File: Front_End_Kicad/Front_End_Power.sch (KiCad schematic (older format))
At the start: 26 parts, among them J201 Conn_01x01_Male, J202 Barrel_Jack, J203 Conn_01x01_Male, SW201 SW_DIP_x01, U201 MAX871, U202 AZ1117IH-5.0TRG1

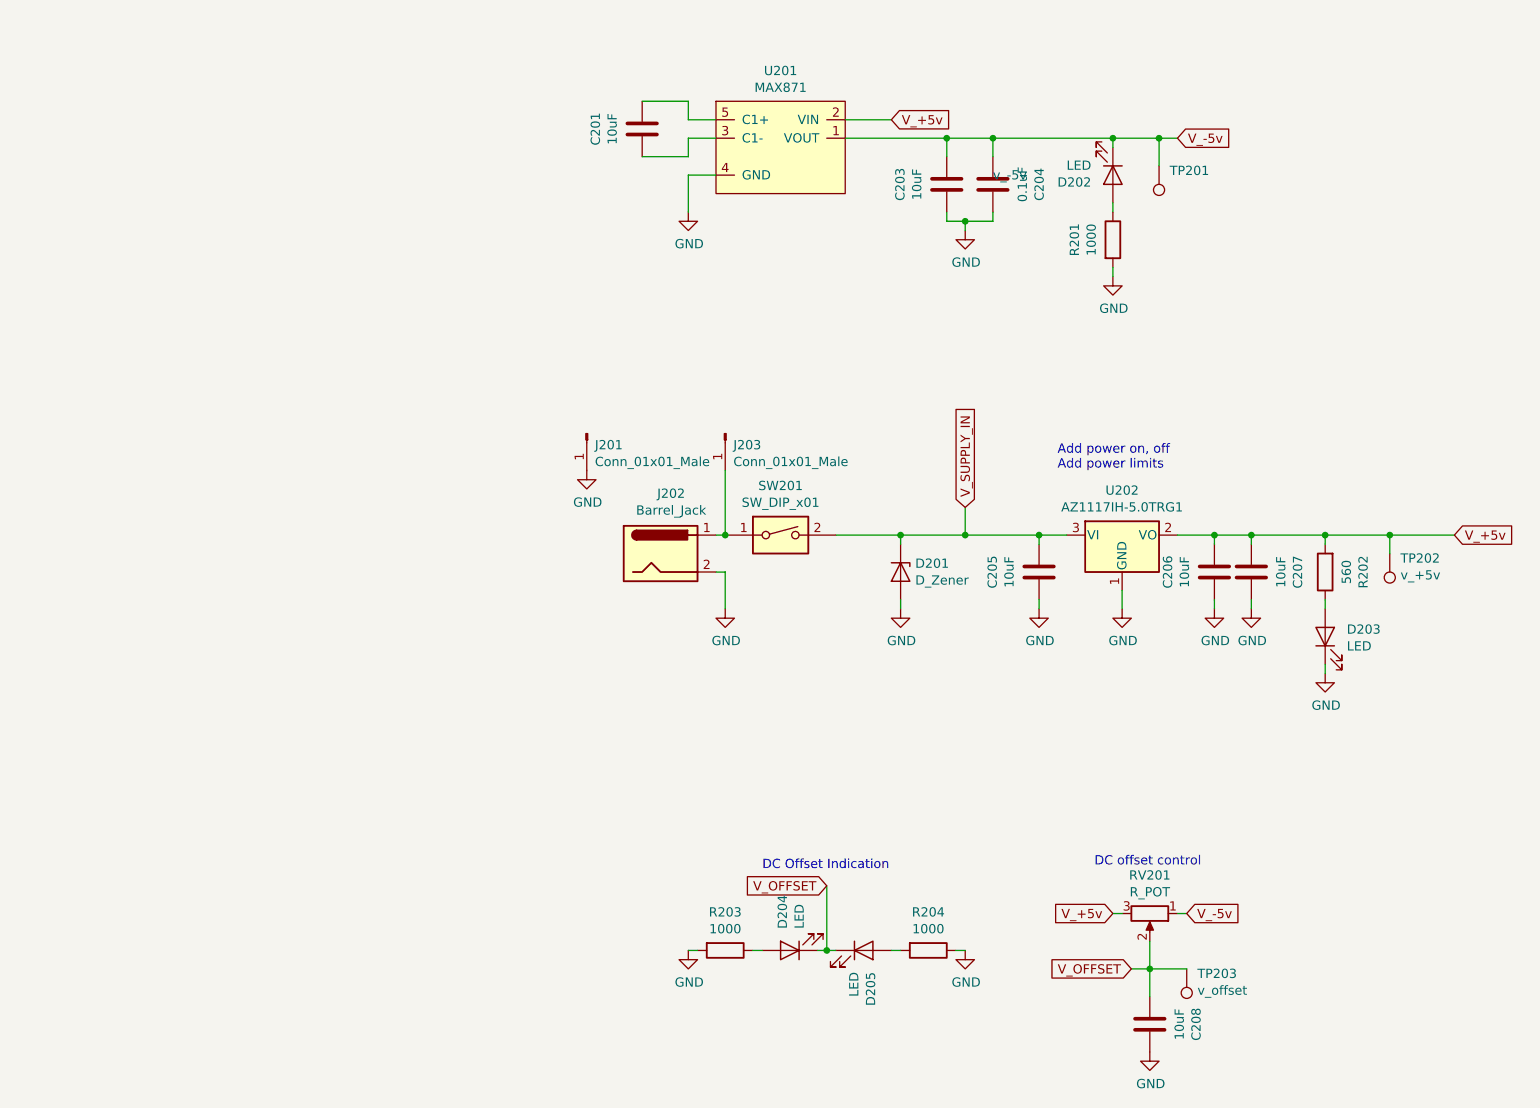
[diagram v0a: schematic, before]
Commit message: Updated schematic
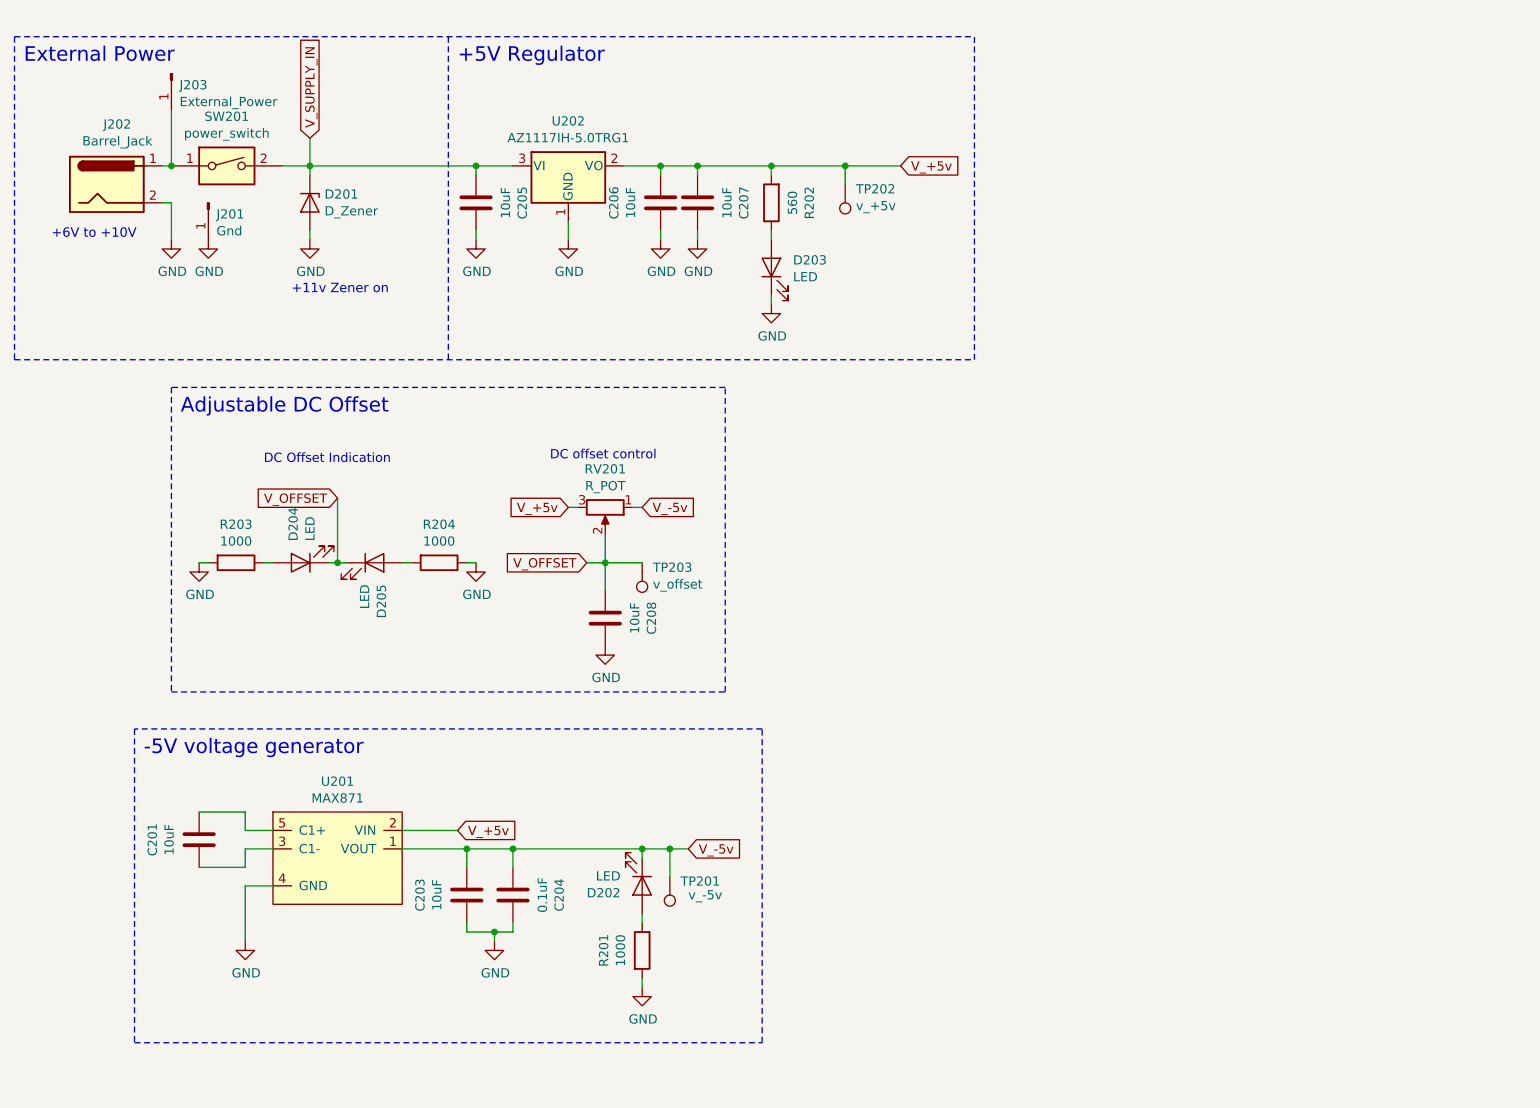
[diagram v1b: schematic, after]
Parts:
- D204, D205: part_name LED Green -> LED Red; part_url https://www.digikey.com/en/products/detail/w%C3%BCrth-elektronik/150120GS75000/4489936 -> https://www.digikey.com/en/products/detail/w%C3%BCrth-elektronik/156120RS75000/4490056
- J201: value Conn_01x01_Male -> Gnd
- J203: value Conn_01x01_Male -> External_Power
- SW201: value SW_DIP_x01 -> power_switch
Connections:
- net GND: now also C205.2; no longer C205.1
- net V_SUPPLY_IN: now also C205.1; no longer C205.2
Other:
- note added: "+11v Zener on"
- note added: "+5V Regulator"
- note added: "+6V to +10V"
- note added: "-5V voltage generator"
- note added: "Adjustable DC Offset"
- note added: "External Power\n"
- note removed: "Add power on, off\nAdd power limits"
- moved on the sheet: C201, C203, C204, C205, C206, C207, C208, D201, D202, D203, D204, D205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
